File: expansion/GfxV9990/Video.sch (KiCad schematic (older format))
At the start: 42 parts, among them J3 S-Video, J4 Composite, J5 RGB Video, J6 Audio In, Q1 2N3904, U6 74HCT04, U7 CXA2075M, Y2 4.4336161875Mhz

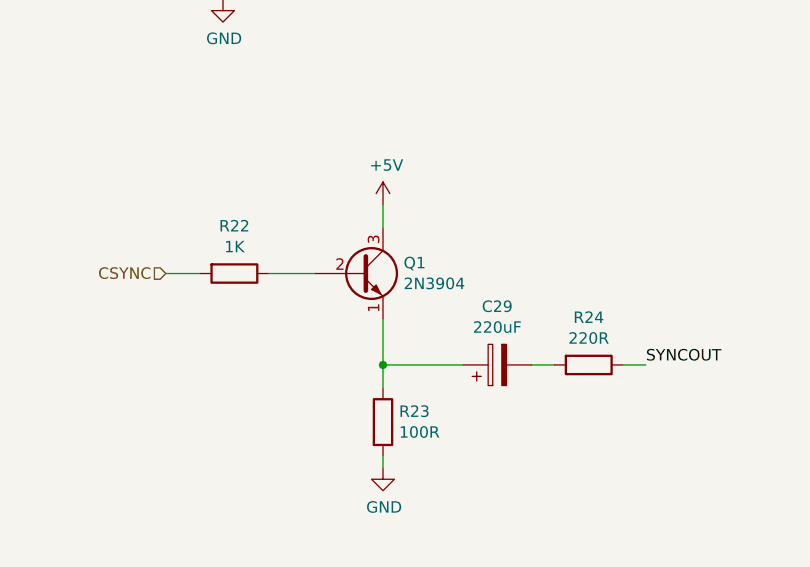
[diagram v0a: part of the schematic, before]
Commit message: Working on video board
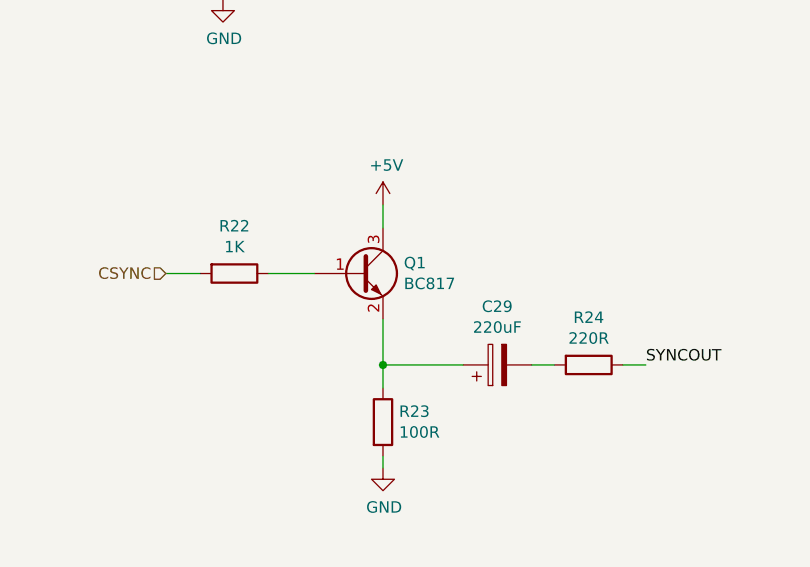
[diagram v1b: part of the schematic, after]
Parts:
- removed Q1: 2N3904, Package_TO_SOT_THT:TO-92_Inline, symbol Transistor_BJT:2N3904
- added Q1: BC817, Package_TO_SOT_SMD:SOT-23, symbol Transistor_BJT:BC817
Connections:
- net +5V: now also Q1.3 (C)
- net at R22.1: now also Q1.1 (B)
- net at C29.1, R23.1: now also Q1.2 (E)
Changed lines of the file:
@@
-$EndComp
-$Comp
-L Transistor_BJT:2N3904 Q1
-U 1 1 60EAD7FF
-P 7000 4750
-F 0 "Q1" H 7190 4796 50  0000 L CNN
-F 1 "2N3904" H 7190 4705 50  0000 L CNN
-F 2 "Package_TO_SOT_THT:TO-92_Inline" H 7200 4675 50  0001 L CIN
-F 3 "https://www.onsemi.com/pub/Collateral/2N3903-D.PDF" H 7000 4750 50  0001 L CNN
-	1    7000 4750
-	1    0    0    -1
 $EndComp
 $Comp
@@
 Wire Wire Line
 	3400 7150 3400 7100
+$Comp
+L Transistor_BJT:BC817 Q1
+U 1 1 60DD58F4
+P 7000 4750
+F 0 "Q1" H 7191 4796 50  0000 L CNN
+F 1 "BC817" H 7191 4705 50  0000 L CNN
+F 2 "Package_TO_SOT_SMD:SOT-23" H 7200 4675 50  0001 L CIN
+F 3 "https://www.onsemi.com/pub/Collateral/BC818-D.pdf" H 7000 4750 50  0001 L CNN
+	1    7000 4750
+	1    0    0    -1
+$EndComp
 $EndSCHEMATC
